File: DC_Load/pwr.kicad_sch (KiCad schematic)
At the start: 52 parts, among them Q1 FDP61N20, Q2 FDP61N20, Q3 FDP61N20, Q4 FDP61N20, Q5 FDP61N20, Q6 FDP61N20, Q7 FDP61N20, Q8 FDP61N20, U1 MCP6034, U5 MCP6034, U7 MCP6034, U8 MCP6034

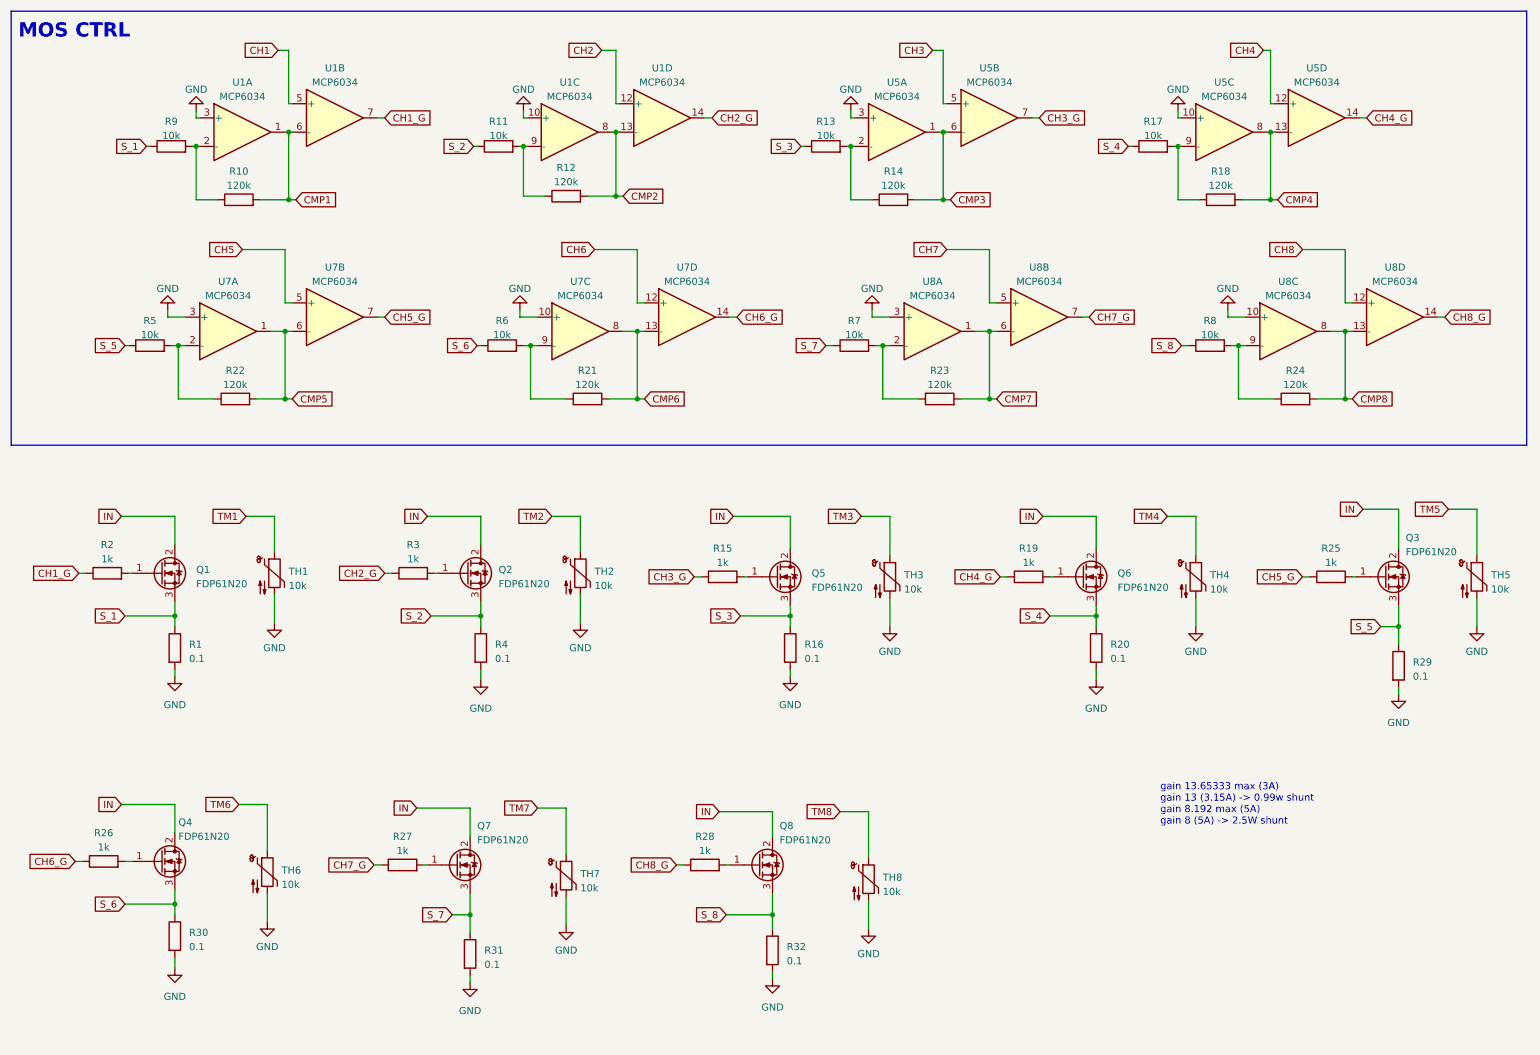
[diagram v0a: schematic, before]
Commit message: Add files via upload
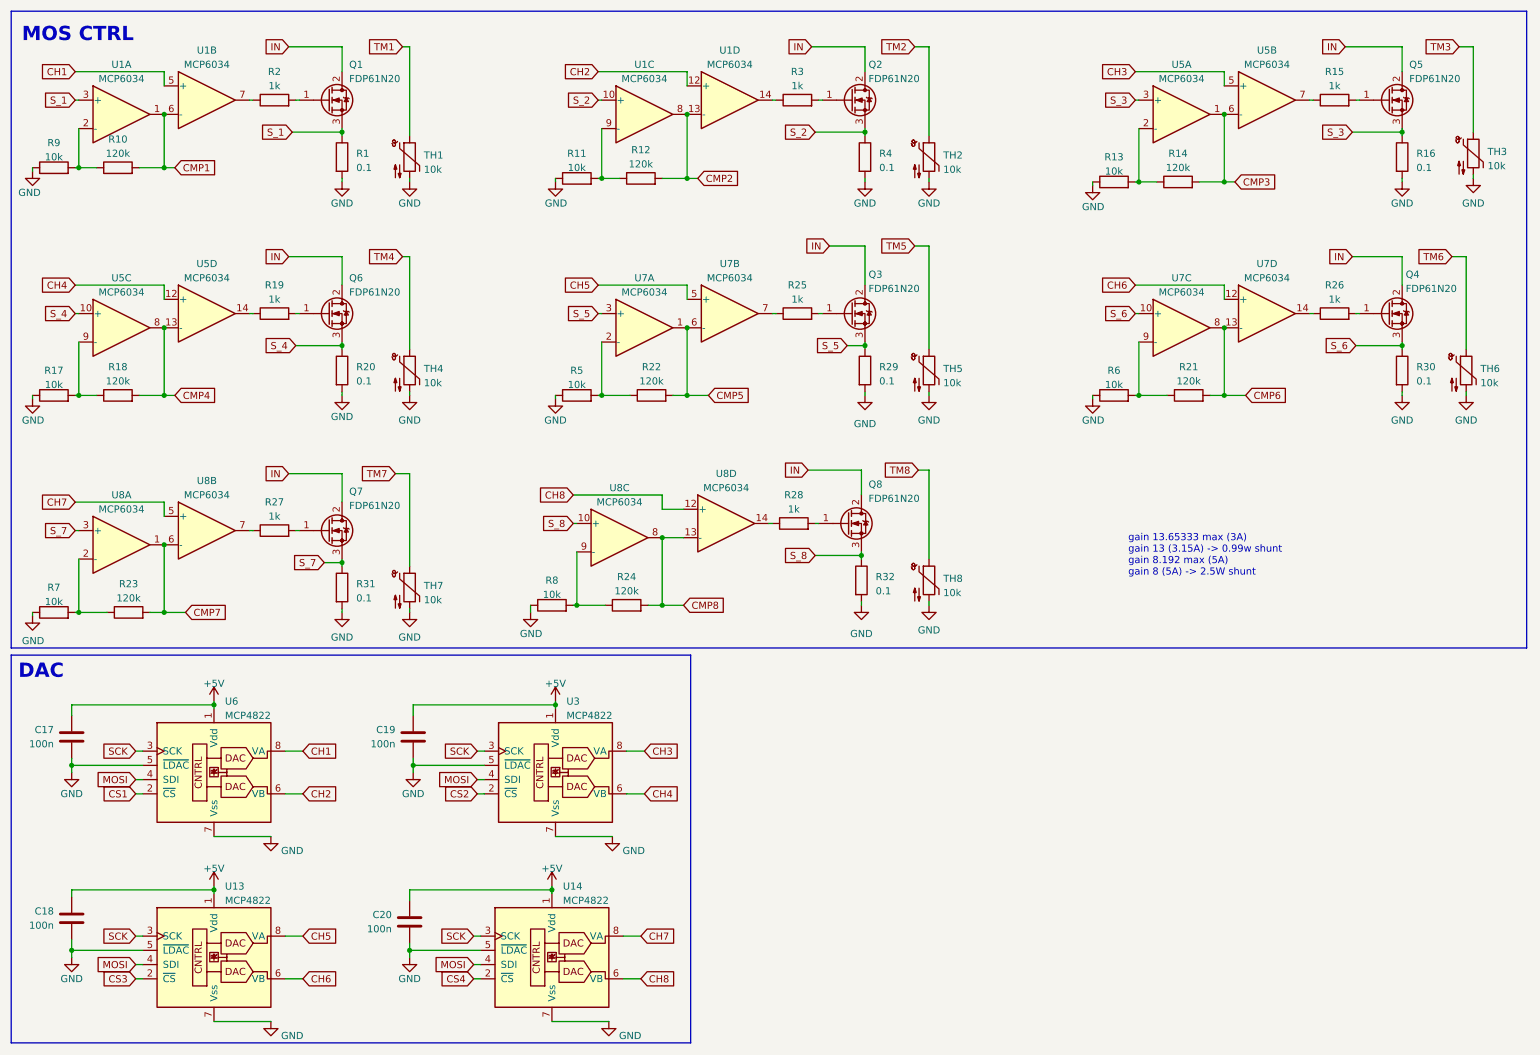
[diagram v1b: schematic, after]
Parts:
- added C17, C18, C19, C20: 100n, symbol Device:C
- added U13, U14, U3, U6: MCP4822, symbol Analog_DAC:MCP4822
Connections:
- net CH1: now also U6.8 (VA)
- net CH2: now also U6.6 (VB)
- net CH3: now also U3.8 (VA)
- net CH4: now also U3.6 (VB)
- net CH5: now also U13.8 (VA)
- net CH6: now also U13.6 (VB)
- net CH7: now also U14.8 (VA)
- net CH8: now also U14.6 (VB)
- net GND: now also R11.1, R13.1, R17.1, R5.1, R6.1, R7.1, R8.1, R9.1, C17.2, C18.2, C19.2, C20.2, U13.5 (~{LDAC}), U13.7 (Vss), U14.5 (~{LDAC}), U14.7 (Vss), U3.5 (~{LDAC}), U3.7 (Vss), U6.5 (~{LDAC}), U6.7 (Vss); no longer U1.10 (+), U1.3 (+), U5.10 (+), U5.3 (+), U7.10 (+), U7.3 (+), U8.10 (+), U8.3 (+)
- net S_1: now also U1.3 (+); no longer R9.1
- net S_2: now also U1.10 (+); no longer R11.1
- net S_3: now also U5.3 (+); no longer R13.1
- net S_4: now also U5.10 (+); no longer R17.1
- net S_5: now also U7.3 (+); no longer R5.1
- net S_6: now also U7.10 (+); no longer R6.1
- net S_7: now also U8.3 (+); no longer R7.1
- net S_8: now also U8.10 (+); no longer R8.1
- net CH1_G: no longer names the net of R2.1, U1.7
- net CH2_G: no longer names the net of R3.1, U1.14
- net CH3_G: no longer names the net of R15.1, U5.7
- net CH4_G: no longer names the net of R19.1, U5.14
- net CH5_G: no longer names the net of R25.1, U7.7
- net CH6_G: no longer names the net of R26.1, U7.14
- net CH7_G: no longer names the net of R27.1, U8.7
- net CH8_G: no longer names the net of R28.1, U8.14
- new net +5V: C17.1, C18.1, C19.1, C20.1, U13.1 (Vdd), U14.1 (Vdd), U3.1 (Vdd), U6.1 (Vdd)
- new net CS1: U6.2 (~{CS})
- new net CS2: U3.2 (~{CS})
- new net CS3: U13.2 (~{CS})
- new net CS4: U14.2 (~{CS})
- new net MOSI: U13.4 (SDI), U14.4 (SDI), U3.4 (SDI), U6.4 (SDI)
- new net SCK: U13.3 (SCK), U14.3 (SCK), U3.3 (SCK), U6.3 (SCK)
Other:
- note added: "DAC"
- moved on the sheet: Q1, Q2, Q3, Q4, Q5, Q6, Q7, Q8, R1, R10, R11, R12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

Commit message: Add files via upload
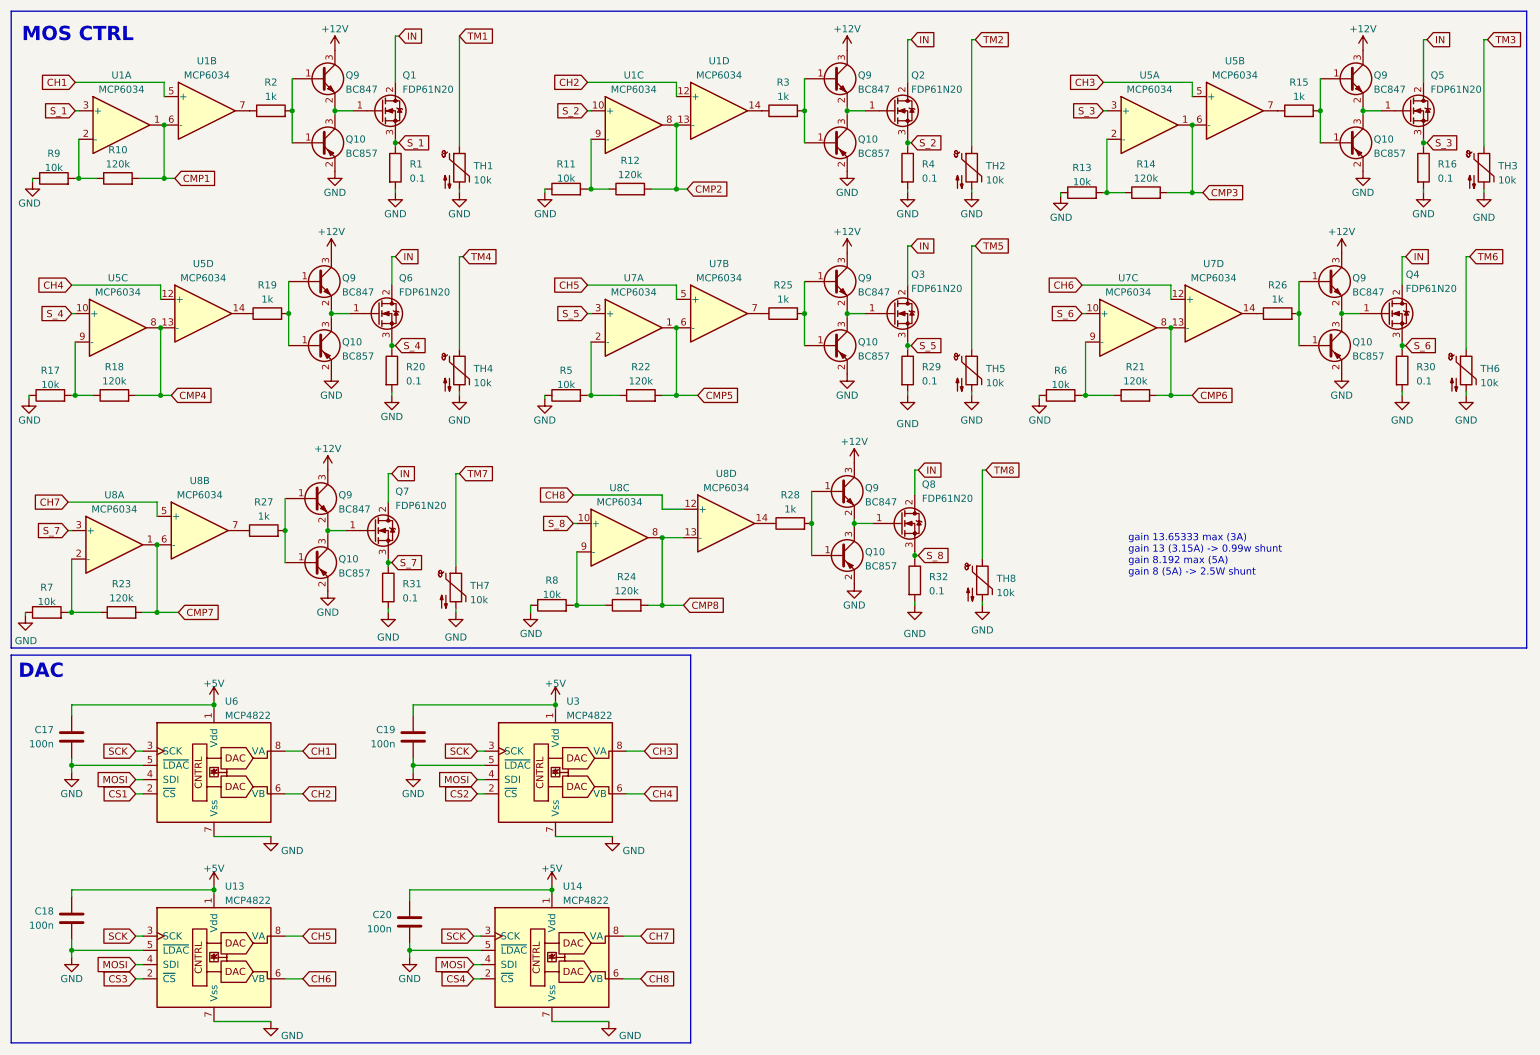
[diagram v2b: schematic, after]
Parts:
- added Q10 (x8): BC857, Package_TO_SOT_SMD:SOT-23, symbol Transistor_BJT:BC857
- added Q9 (x8): BC847, Package_TO_SOT_SMD:SOT-23, symbol Transistor_BJT:BC847
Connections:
- net GND: now also Q10.2 (E), Q10.2 (E), Q10.2 (E), Q10.2 (E), Q10.2 (E), Q10.2 (E), Q10.2 (E), Q10.2 (E)
- net at R26.2: now also Q10.1 (B), Q9.1 (B); no longer Q4.1 (G)
- net at Q5.1 (G): now also Q10.3 (C), Q9.2 (E); no longer R15.2
- net at R19.2: now also Q10.1 (B), Q9.1 (B); no longer Q6.1 (G)
- net at Q3.1 (G): now also Q10.3 (C), Q9.2 (E); no longer R25.2
- net at R27.2: now also Q10.1 (B), Q9.1 (B); no longer Q7.1 (G)
- net at R3.2: now also Q10.1 (B), Q9.1 (B); no longer Q2.1 (G)
- net at R28.2: now also Q10.1 (B), Q9.1 (B); no longer Q8.1 (G)
- net at R2.2: now also Q10.1 (B), Q9.1 (B); no longer Q1.1 (G)
- new net: Q10.3 (C), Q8.1 (G), Q9.2 (E)
- new net: Q10.3 (C), Q7.1 (G), Q9.2 (E)
- new net: Q10.3 (C), Q4.1 (G), Q9.2 (E)
- new net: Q10.3 (C), Q2.1 (G), Q9.2 (E)
- new net: Q1.1 (G), Q10.3 (C), Q9.2 (E)
- new net: Q10.1 (B), Q9.1 (B), R25.2
- new net: Q10.3 (C), Q6.1 (G), Q9.2 (E)
- new net: Q10.1 (B), Q9.1 (B), R15.2
- new net +12V: Q9.3 (C), Q9.3 (C), Q9.3 (C), Q9.3 (C), Q9.3 (C), Q9.3 (C), Q9.3 (C), Q9.3 (C)
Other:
- moved on the sheet: Q1, Q2, Q3, Q5, Q6, Q7, Q8, R1, R10, R11, R12, R13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
